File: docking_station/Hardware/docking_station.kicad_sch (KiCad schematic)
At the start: 56 parts, among them IC1 VOM1271T, IC2 VOM1271T, IC3 VOM1271T, IC4 VOM1271T, IC5 VOM1271T, J1 SUPPLY_EN, J2 LIVE_IN, J5 SUPPLY+, J6 SUPPLY-, K1 RELPOL R40N-3021-85-1024, K2 EC2-3NU, K3 EC2-3NU, Q1 SIDR392DP-T1-GE3, Q10 DN2540N8-G, Q11 DN2540N8-G, Q2 SIDR392DP-T1-GE3, Q3 SIDR392DP-T1-GE3, Q4 SIDR392DP-T1-GE3, Q5 SIDR392DP-T1-GE3, Q6 SIDR392DP-T1-GE3, Q7 SIDR392DP-T1-GE3, Q8 SIDR392DP-T1-GE3, Q9 SIDR392DP-T1-GE3, U1 LTC4357MS8, U2 Comparator, U3 L78L05AB, U4 ACS712xLCTR-20A, U5 LMV321IYLT, U6 Comparator

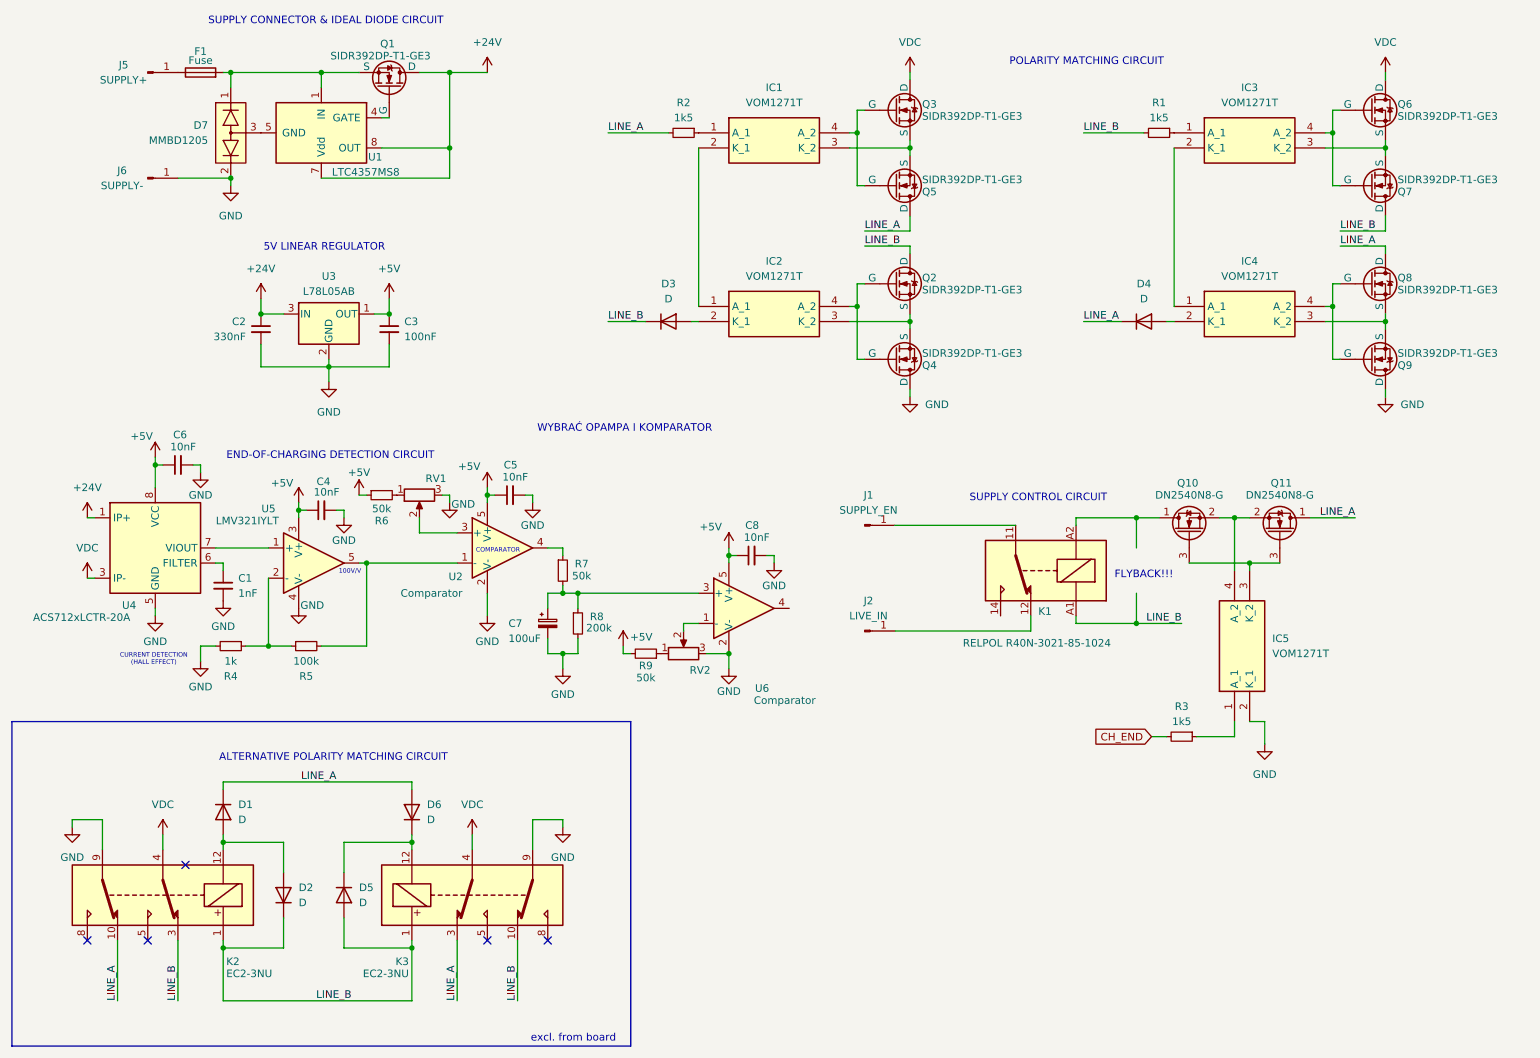
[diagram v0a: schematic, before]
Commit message: almost done
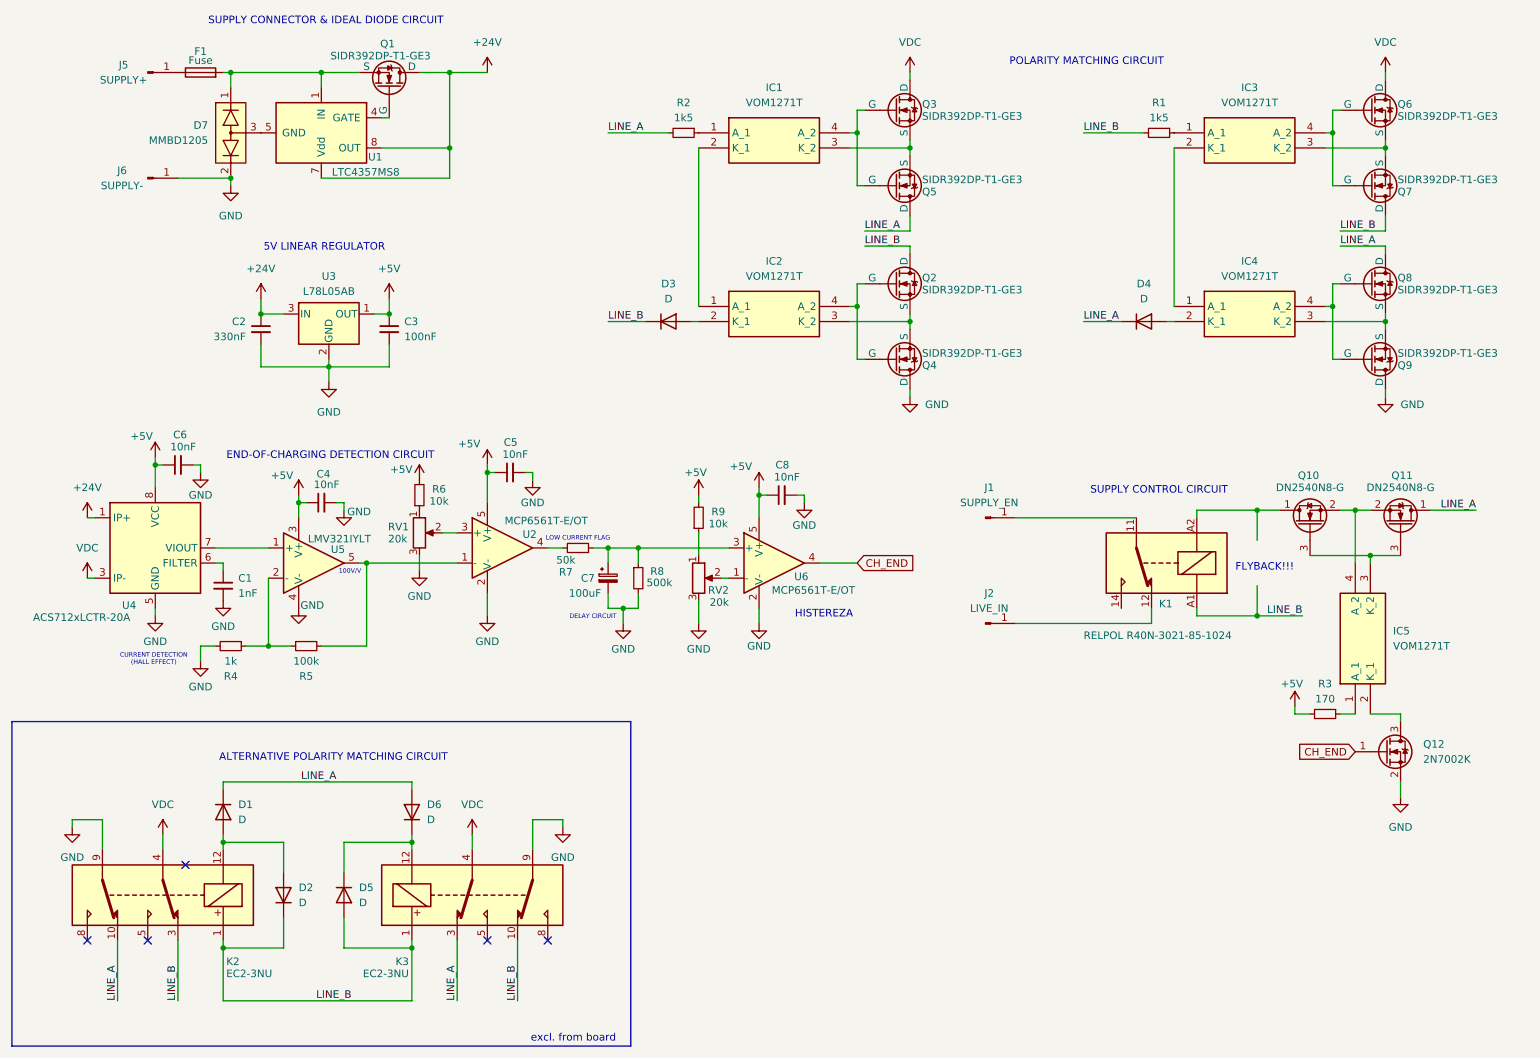
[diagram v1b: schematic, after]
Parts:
- added Q12: 2N7002K, Package_TO_SOT_SMD:SOT-23, symbol Transistor_FET:2N7002K
- R3: value 1k5 -> 170
- R6, R9: value 50k -> 10k
- R8: value 200k -> 500k
- RV1, RV2: value R_Potentiometer -> 20k
- U2, U6: value Comparator -> MCP6561T-E/OT
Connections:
- net +5V: now also R3.2, R6.2; no longer R6.1
- net CH_END: now also U6.4, Q12.1 (G); no longer R3.2
- net GND: now also Q12.2 (S); no longer IC5.2 (K_1)
- net at C7.1, R8.1, U6.3 (+): now also R7.1; no longer R7.2
- net at U2.4: now also R7.2; no longer R7.1
- net at RV1.1: now also R6.1; no longer R6.2
- new net: IC5.2 (K_1), Q12.3 (D)
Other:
- note added: "DELAY CIRCUIT"
- note added: "HISTEREZA"
- note added: "LOW CURRENT FLAG"
- note removed: "COMPARATOR"
- note removed: "WYBRAĆ OPAMPA I KOMPARATOR"
- moved on the sheet: C4, C5, C7, C8, IC5, J1, J2, K1, Q10, Q11, R3, R8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
